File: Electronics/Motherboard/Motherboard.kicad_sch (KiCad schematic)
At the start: 54 parts, among them J1 DX07S024JJ3R1300, M1 AO3400A, M2 AO3400A, M3 AO3400A, U1 AMS1117-3.3, U2 TMC2209_SILENTSTEPSTICK, U3 TMC2209_SILENTSTEPSTICK, U4 TMC2209_SILENTSTEPSTICK, U5 TMC2209_SILENTSTEPSTICK, U6 LM2576HVS-5, U7 STM32G0B1VETx

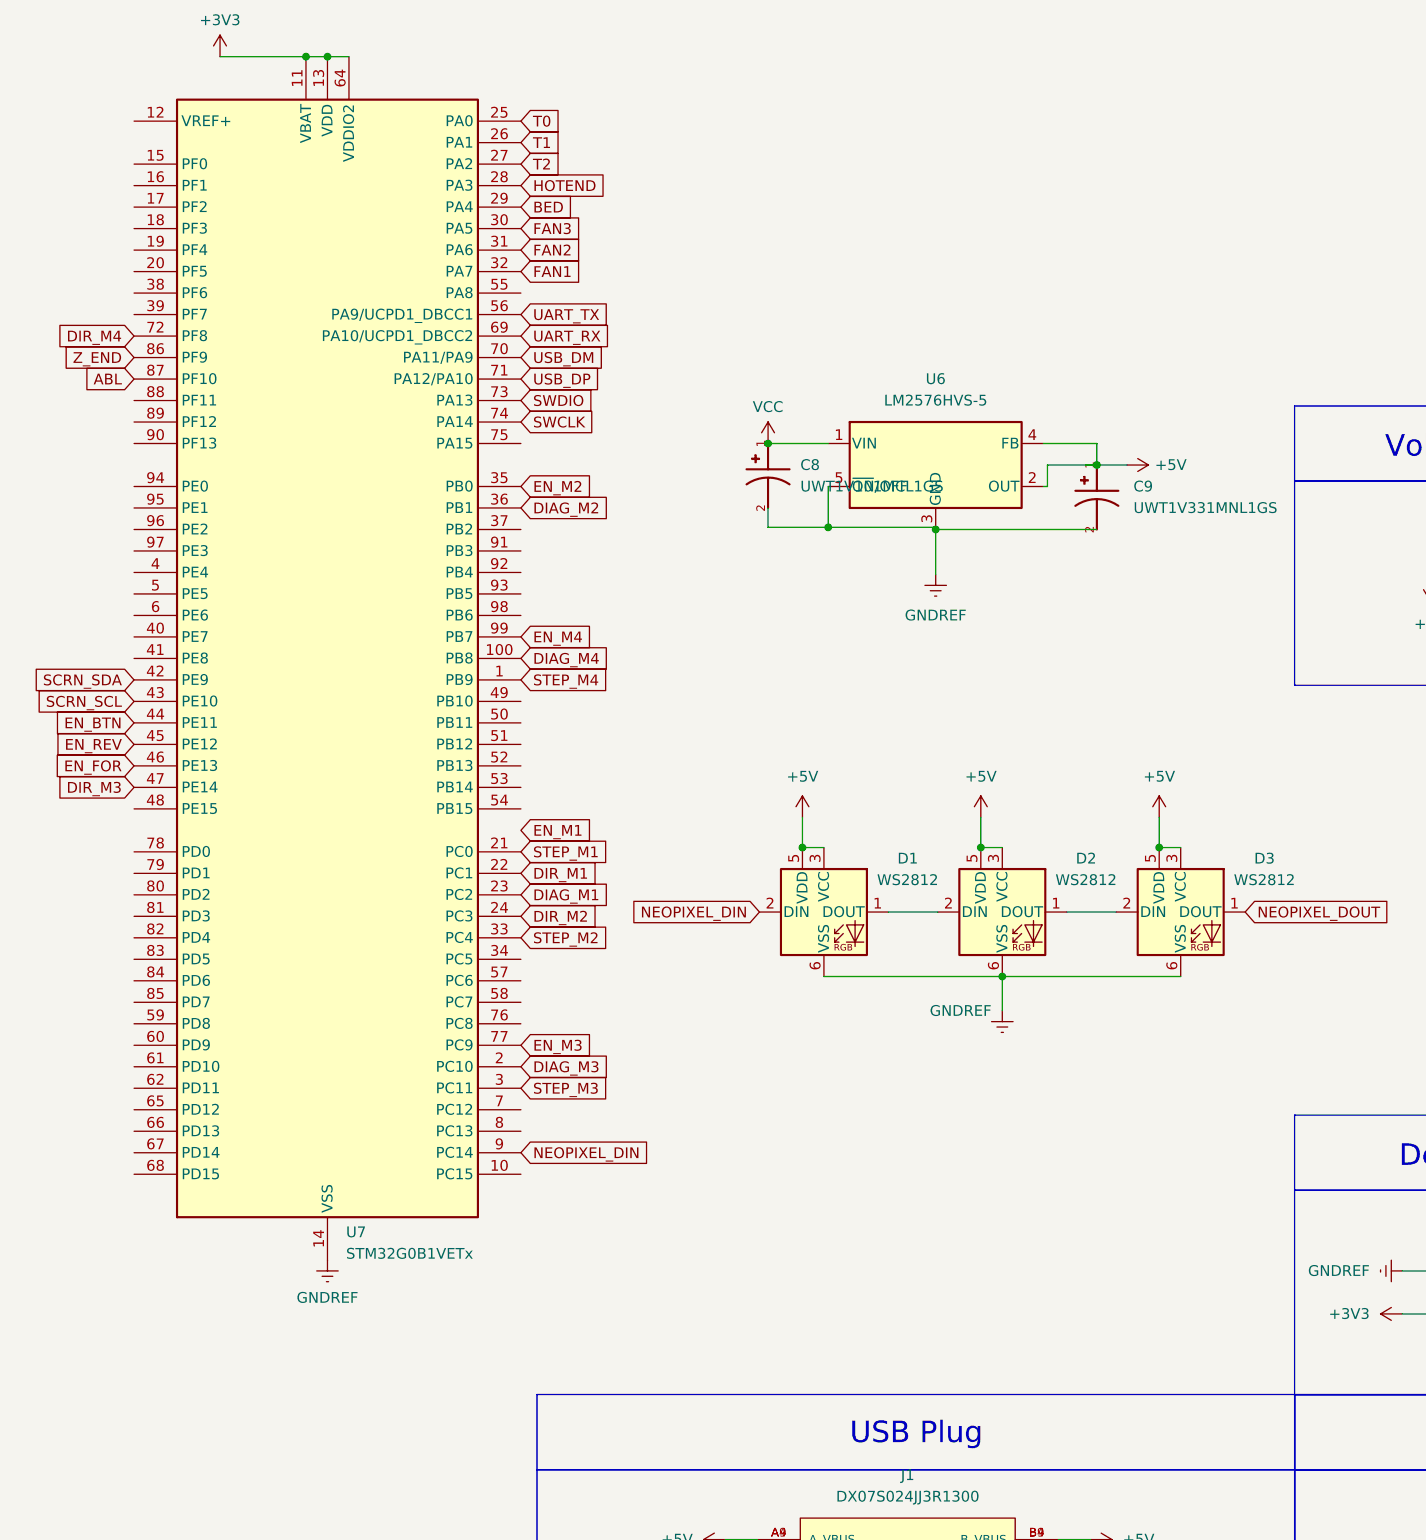
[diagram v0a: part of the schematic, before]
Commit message: so i kinda added an extra thing for more IO uhhhhhhhh
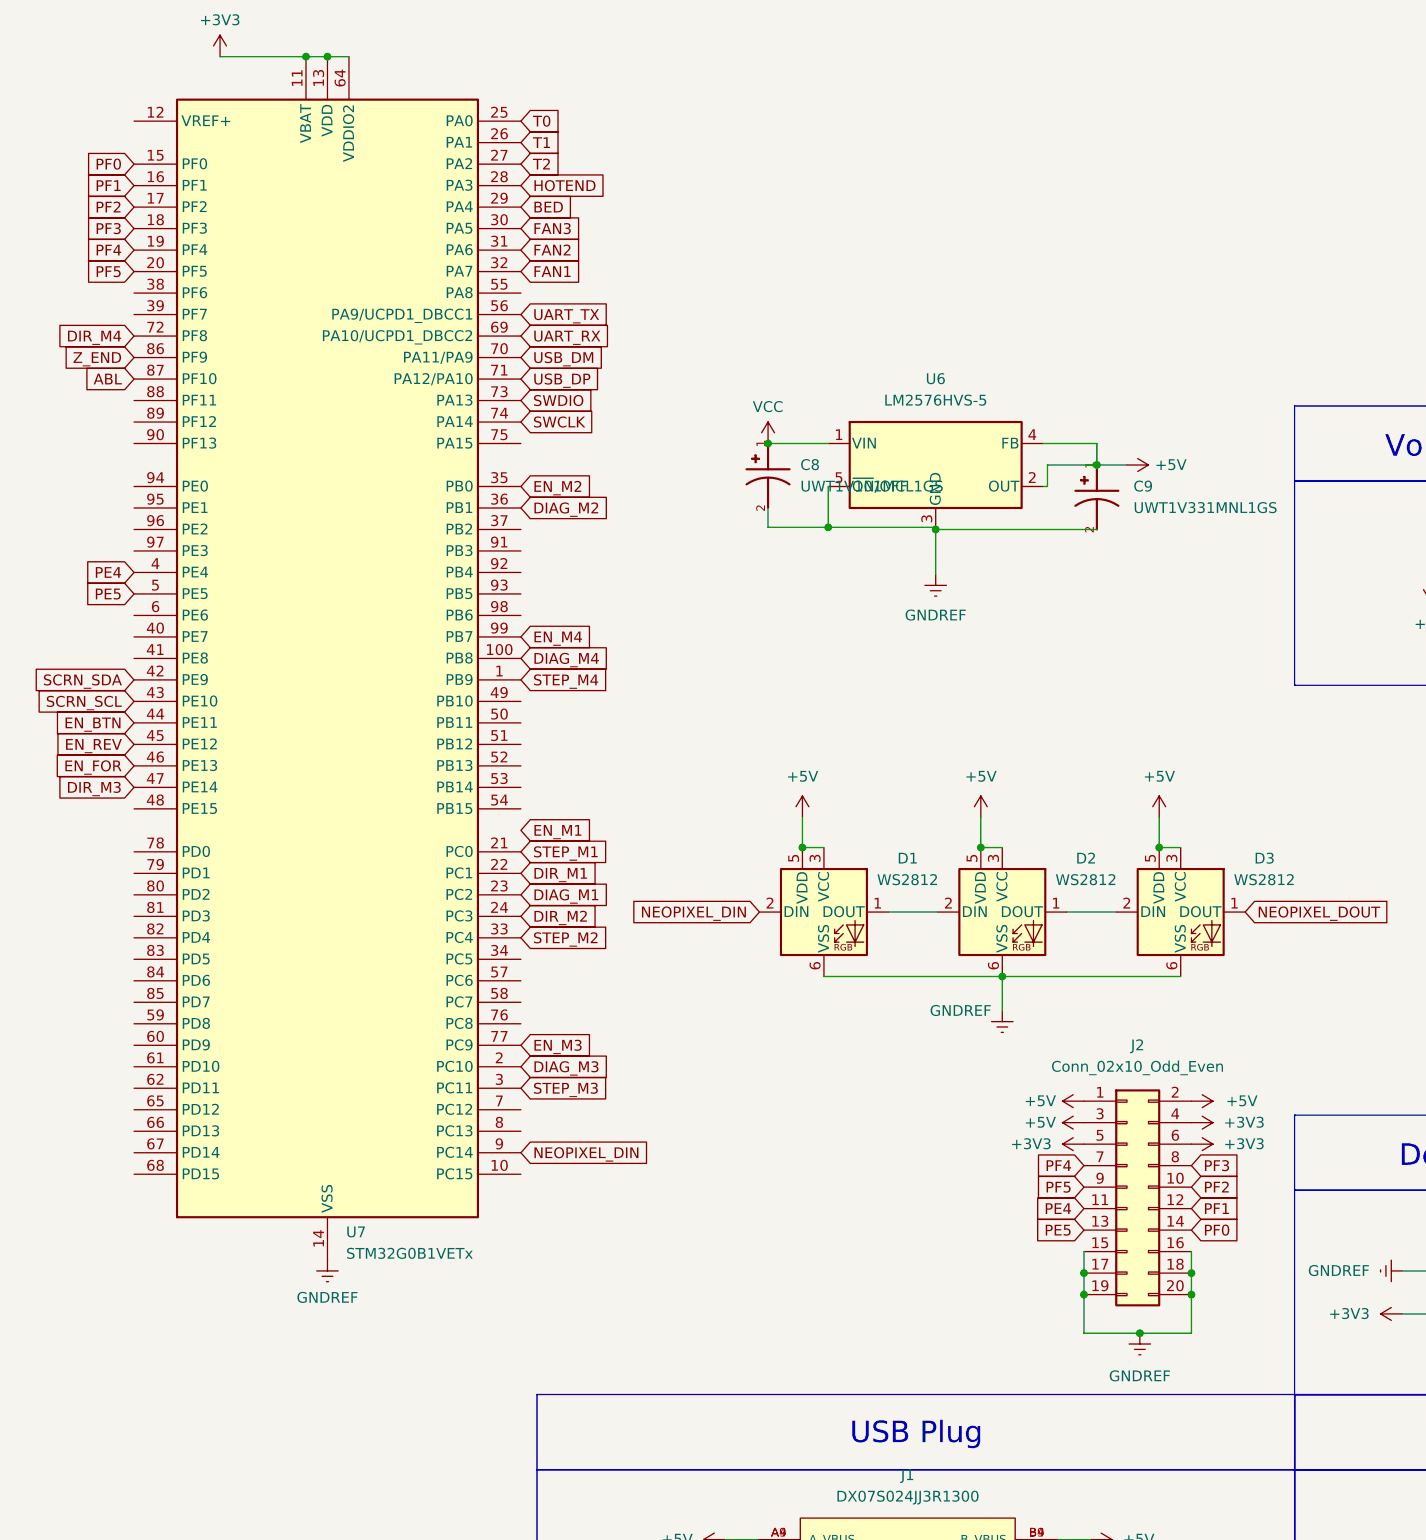
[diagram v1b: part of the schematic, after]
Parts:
- added J2: Conn_02x10_Odd_Even, 2x10_tht:PinBox-2.54-02x10-THT, symbol Connector_Generic:Conn_02x10_Odd_Even
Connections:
- net +3V3: now also J2.4 (Pin_4), J2.5 (Pin_5), J2.6 (Pin_6)
- net +5V: now also J2.1 (Pin_1), J2.2 (Pin_2), J2.3 (Pin_3)
- net GNDREF: now also J2.15 (Pin_15), J2.16 (Pin_16), J2.17 (Pin_17), J2.18 (Pin_18), J2.19 (Pin_19), J2.20 (Pin_20)
- net PF0: now reaches U7.15 (PF0)
- net PF0: now also J2.14 (Pin_14)
- net PF1: now reaches U7.16 (PF1)
- net PF1: now also J2.12 (Pin_12)
- net PF2: now reaches U7.17 (PF2)
- net PF2: now also J2.10 (Pin_10)
- net PF3: now reaches U7.18 (PF3)
- net PF3: now also J2.8 (Pin_8)
- net PF4: now reaches U7.19 (PF4)
- net PF4: now also J2.7 (Pin_7)
- net PF5: now reaches U7.20 (PF5)
- net PF5: now also J2.9 (Pin_9)
- net PE4: now reaches U7.4 (PE4)
- net PE4: now also J2.11 (Pin_11)
- net PE5: now reaches U7.5 (PE5)
- net PE5: now also J2.13 (Pin_13)
